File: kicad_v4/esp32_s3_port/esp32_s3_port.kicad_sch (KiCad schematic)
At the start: 51 parts, among them J1 AudioJack4, J2 AudioJack4, SW1 KS33_SW_HS, SW10 KS33_SW_HS, SW11 KS33_SW_HS, SW12 KS33_SW_HS, SW13 KS33_SW_HS, SW14 KS33_SW_HS, SW15 KS33_SW_HS, SW16 KS33_SW_HS, SW17 KS33_SW_HS, SW18 KS33_SW_HS, SW19 KS33_SW_HS, SW2 KS33_SW_HS, SW20 KS33_SW_HS, SW21 KS33_SW_HS, SW22 Slide_Switch_SPDT_P3mm_10x5x1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, SW3 KS33_SW_HS, SW4 KS33_SW_HS, SW5 KS33_SW_HS, SW6 KS33_SW_HS, SW7 KS33_SW_HS, SW8 KS33_SW_HS, SW9 KS33_SW_HS, U1 TP4057

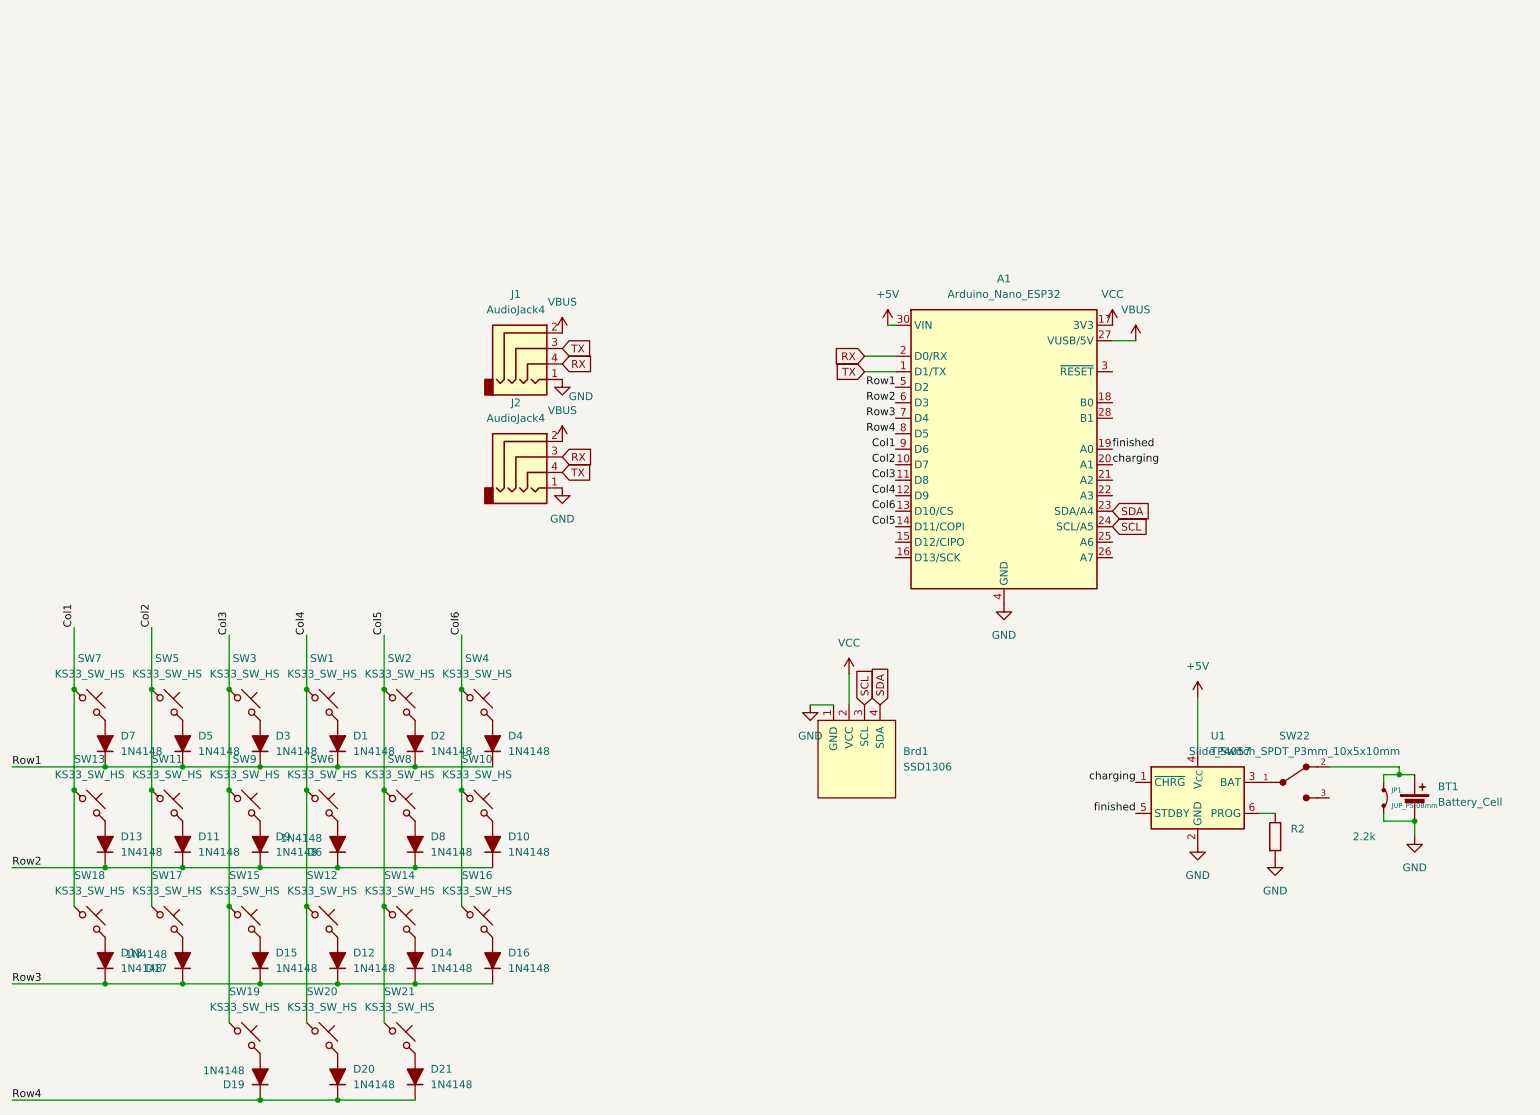
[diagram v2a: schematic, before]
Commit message: updates
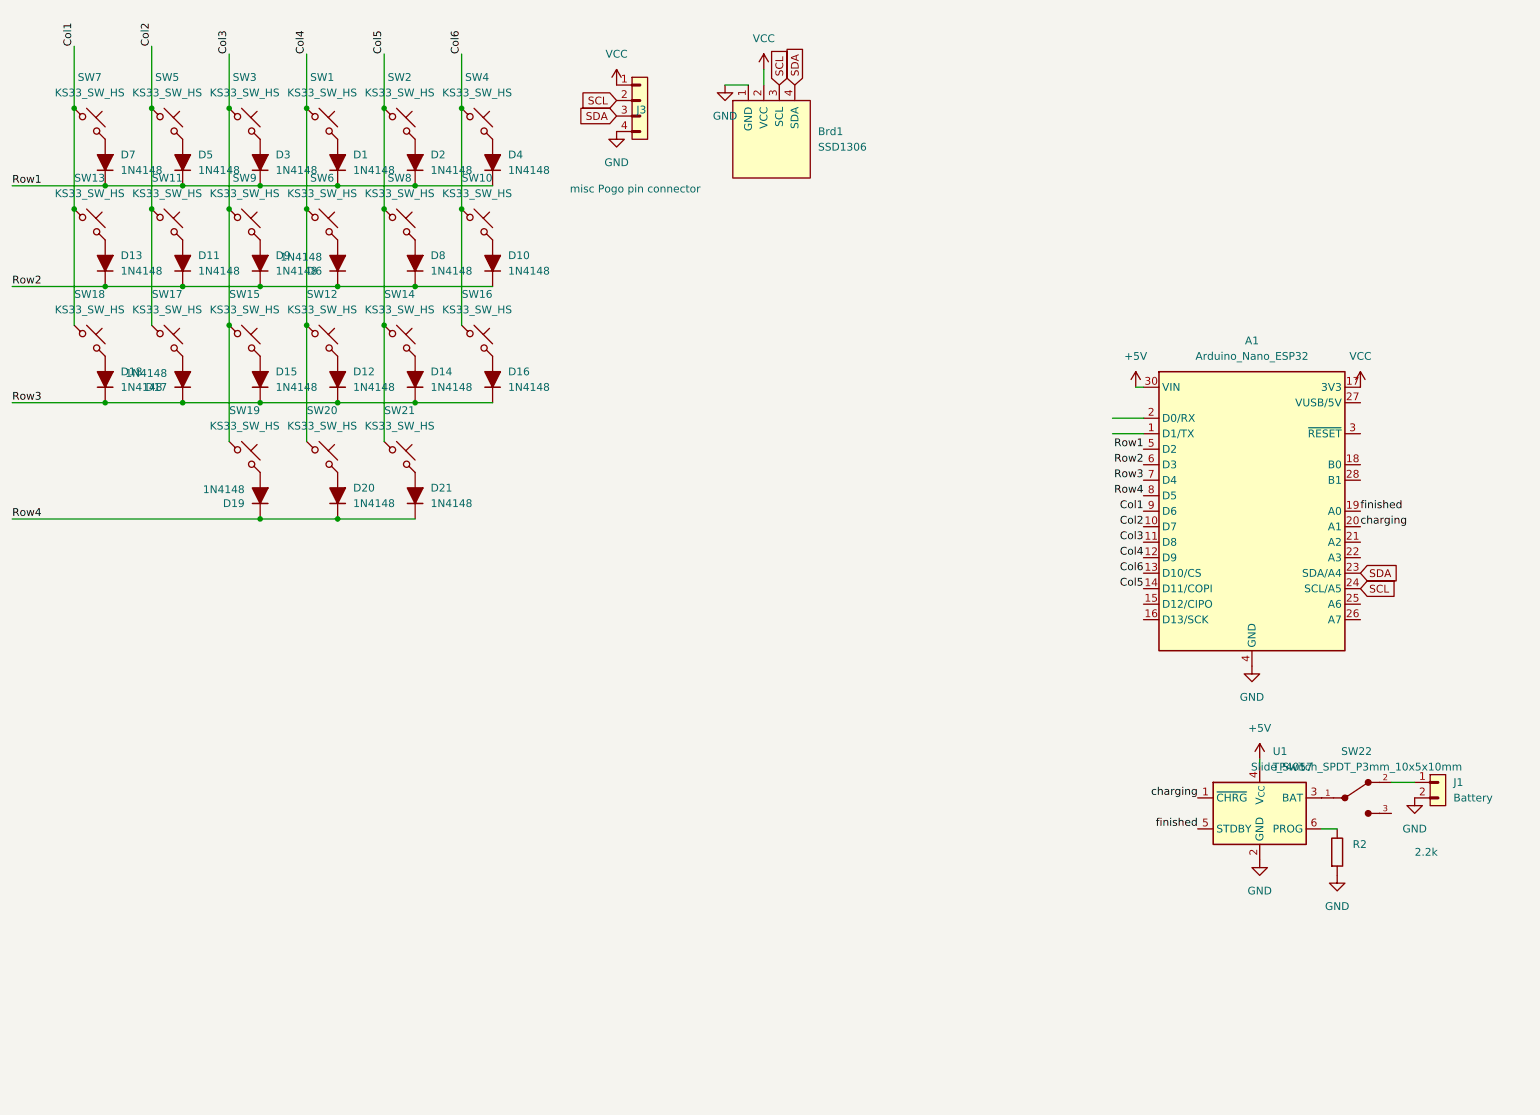
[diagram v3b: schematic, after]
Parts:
- removed BT1: Battery_Cell, symbol Device:Battery_Cell
- removed J1, J2: AudioJack4, PJ-320A_Library:PJ-320A, symbol TRRS:AudioJack4
- removed JP1: JUP_P5.08mm, PCM_SL_Jumpers:JUP_P5.08mm, symbol PCM_SL_Jumpers_THT:JUP_P5.08mm
- added J1: Battery, Connector_PinHeader_2.54mm:PinHeader_1x02_P2.54mm_Vertical, symbol PCM_SL_Pin_Headers:PINHD_1x2_Male
- added J3: misc Pogo pin connector, Connector_PinHeader_2.54mm:PinHeader_1x04_P2.54mm_Vertical, symbol PCM_SL_Pin_Headers:PINHD_1x4_Male
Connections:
- net GND: now also J1.2, J3.4
- net SCL: now also J3.2
- net SDA: now also J3.3
- net VCC: now also J3.1
- net at SW22.2: now also J1.1
- net RX: no longer names the net of A1.2 (D0/RX)
- net TX: no longer names the net of A1.1 (D1/TX)
- net VBUS: no longer names the net of A1.27 (VUSB/5V)
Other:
- moved on the sheet: A1, Brd1, D1, D10, D11, D12, D13, D14, D15, D16, D17, D18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
